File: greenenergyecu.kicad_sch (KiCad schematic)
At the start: 1 part, among them U1 ICM7555xB

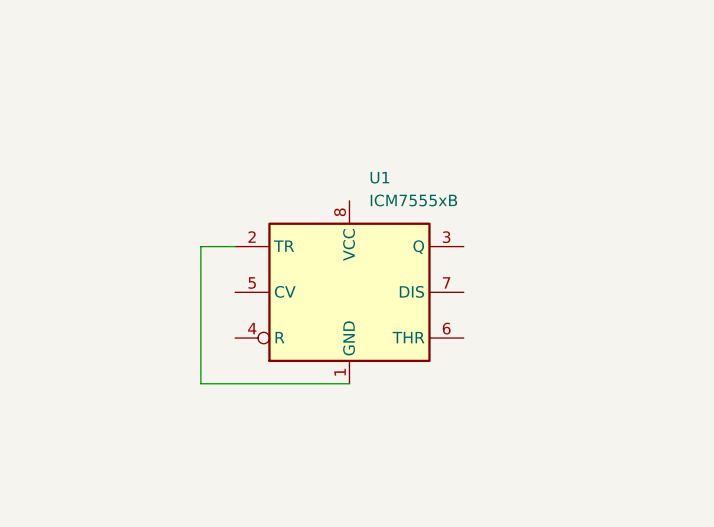
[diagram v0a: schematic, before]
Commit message: rt
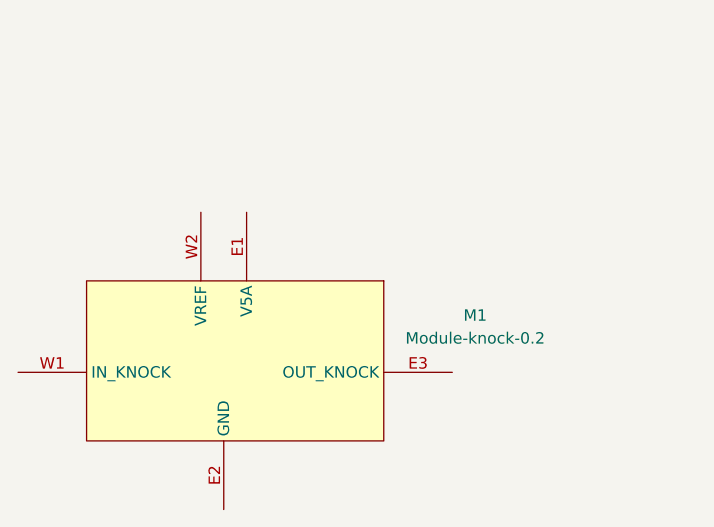
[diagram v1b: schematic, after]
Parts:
- removed U1: ICM7555xB, Package_SO:SOIC-8_3.9x4.9mm_P1.27mm, symbol Timer:ICM7555xB
- added M1: Module-knock-0.2, hellen-one-knock-0.2:knock, symbol knock:Module-knock-0.2
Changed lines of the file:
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@@
 	(generator_version "8.0")
 	(paper "A4")
-	(wire
-		(pts
-			(xy 82.55 82.55) (xy 78.74 82.55)
-		)
-		(stroke
-			(width 0)
-			(type default)
-		)
-	)
-	(wire
-		(pts
-			(xy 78.74 82.55) (xy 78.74 97.79)
-		)
-		(stroke
-			(width 0)
-			(type default)
-		)
-	)
-	(wire
-		(pts
-			(xy 95.25 97.79) (xy 78.74 97.79)
-		)
-		(stroke
-			(width 0)
-			(type default)
-		)
-	)
 	(symbol
-		(lib_id "Timer:ICM7555xB")
-		(at 95.25 87.63 0)
+		(lib_id "knock:Module-knock-0.2")
+		(at 66.04 86.36 0)
 		(unit 1)
 		(exclude_from_sim no)
@@
 		(dnp no)
 		(fields_autoplaced yes)
-		(property "Reference" "U1"
-			(at 97.4441 74.93 0)
+		(property "Reference" "M1"
+			(at 109.22 90.2014 0)
 			(effects
 				(font
 					(size 1.27 1.27)
 				)
-				(justify left)
 			)
 		)
-		(property "Value" "ICM7555xB"
-			(at 97.4441 77.47 0)
+		(property "Value" "Module-knock-0.2"
+			(at 109.22 92.7414 0)
 			(effects
 				(font
 					(size 1.27 1.27)
 				)
-				(justify left)
 			)
 		)
-		(property "Footprint" "Package_SO:SOIC-8_3.9x4.9mm_P1.27mm"
-			(at 116.84 97.79 0)
+		(property "Footprint" "hellen-one-knock-0.2:knock"
+			(at 66.04 86.36 0)
 			(effects
 				(font
@@
 			)
 		)
-		(property "Datasheet" "http://www.intersil.com/content/dam/Intersil/documents/icm7/icm7555-56.pdf"
-			(at 116.84 97.79 0)
+		(property "Datasheet" ""
+			(at 66.04 86.36 0)
 			(effects
 				(font
@@
 			)
 		)
-		(property "Description" "CMOS General Purpose Timer, 555 compatible, SOIC-8"
-			(at 95.25 87.63 0)
+		(property "Description" "Hellen-One Knock Pre-amplifier Module"
+			(at 66.04 86.36 0)
 			(effects
 				(font
@@
 			)
 		)
-		(pin "4"
+		(pin "W1"
 		)
-		(pin "2"
+		(pin "W2"
 		)
-		(pin "5"
+		(pin "E1"
 		)
-		(pin "3"
+		(pin "E2"
 		)
-		(pin "8"
-		)
-		(pin "7"
-		)
-		(pin "6"
-		)
-		(pin "1"
+		(pin "E3"
 		)
 		(instances
 			(project ""
 				(path "/e34f8548-18bd-4553-87dc-fac974a7531b"
-					(reference "U1")
+					(reference "M1")
 					(unit 1)
 				)

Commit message: ee
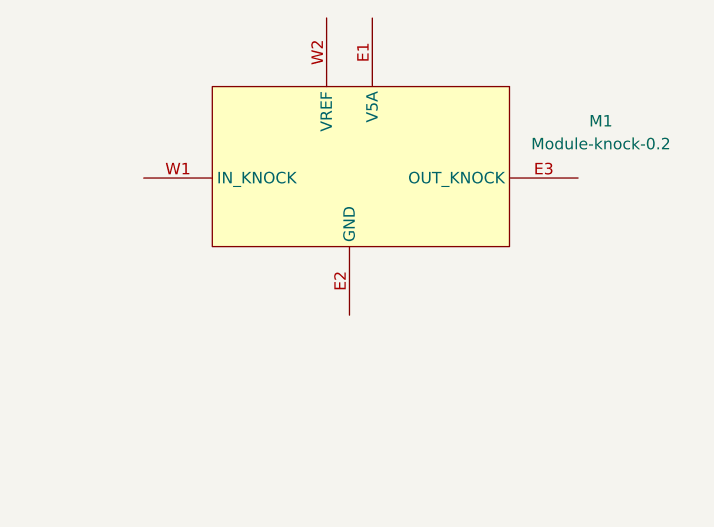
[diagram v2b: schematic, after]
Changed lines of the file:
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@@
 	(symbol
 		(lib_id "knock:Module-knock-0.2")
-		(at 66.04 86.36 0)
+		(at 80.01 64.77 0)
 		(unit 1)
 		(exclude_from_sim no)
@@
 		(fields_autoplaced yes)
 		(property "Reference" "M1"
-			(at 109.22 90.2014 0)
+			(at 123.19 68.6114 0)
 			(effects
 				(font
@@
 		)
 		(property "Value" "Module-knock-0.2"
-			(at 109.22 92.7414 0)
+			(at 123.19 71.1514 0)
 			(effects
 				(font
@@
 		)
 		(property "Footprint" "hellen-one-knock-0.2:knock"
-			(at 66.04 86.36 0)
+			(at 80.01 64.77 0)
 			(effects
 				(font
@@
 		)
 		(property "Datasheet" ""
-			(at 66.04 86.36 0)
+			(at 80.01 64.77 0)
 			(effects
 				(font
@@
 		)
 		(property "Description" "Hellen-One Knock Pre-amplifier Module"
-			(at 66.04 86.36 0)
+			(at 80.01 64.77 0)
 			(effects
 				(font
@@
 			)
 		)
+		(pin "W2"
+		)
+		(pin "E3"
+		)
 		(pin "W1"
-		)
-		(pin "W2"
 		)
 		(pin "E1"
@@
 		(pin "E2"
 		)
-		(pin "E3"
-		)
 		(instances
